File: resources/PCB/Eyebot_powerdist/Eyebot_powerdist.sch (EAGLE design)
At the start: 33 parts, among them IC3 MCP23016SO, K1 62000211622, K2 62000211622, K3 62000211622, K4 62000211622, K5 62000211622, K6 62000211622, K7 61201021621, Q1 2N2222, Q2 2N2222, Q3 2N2222

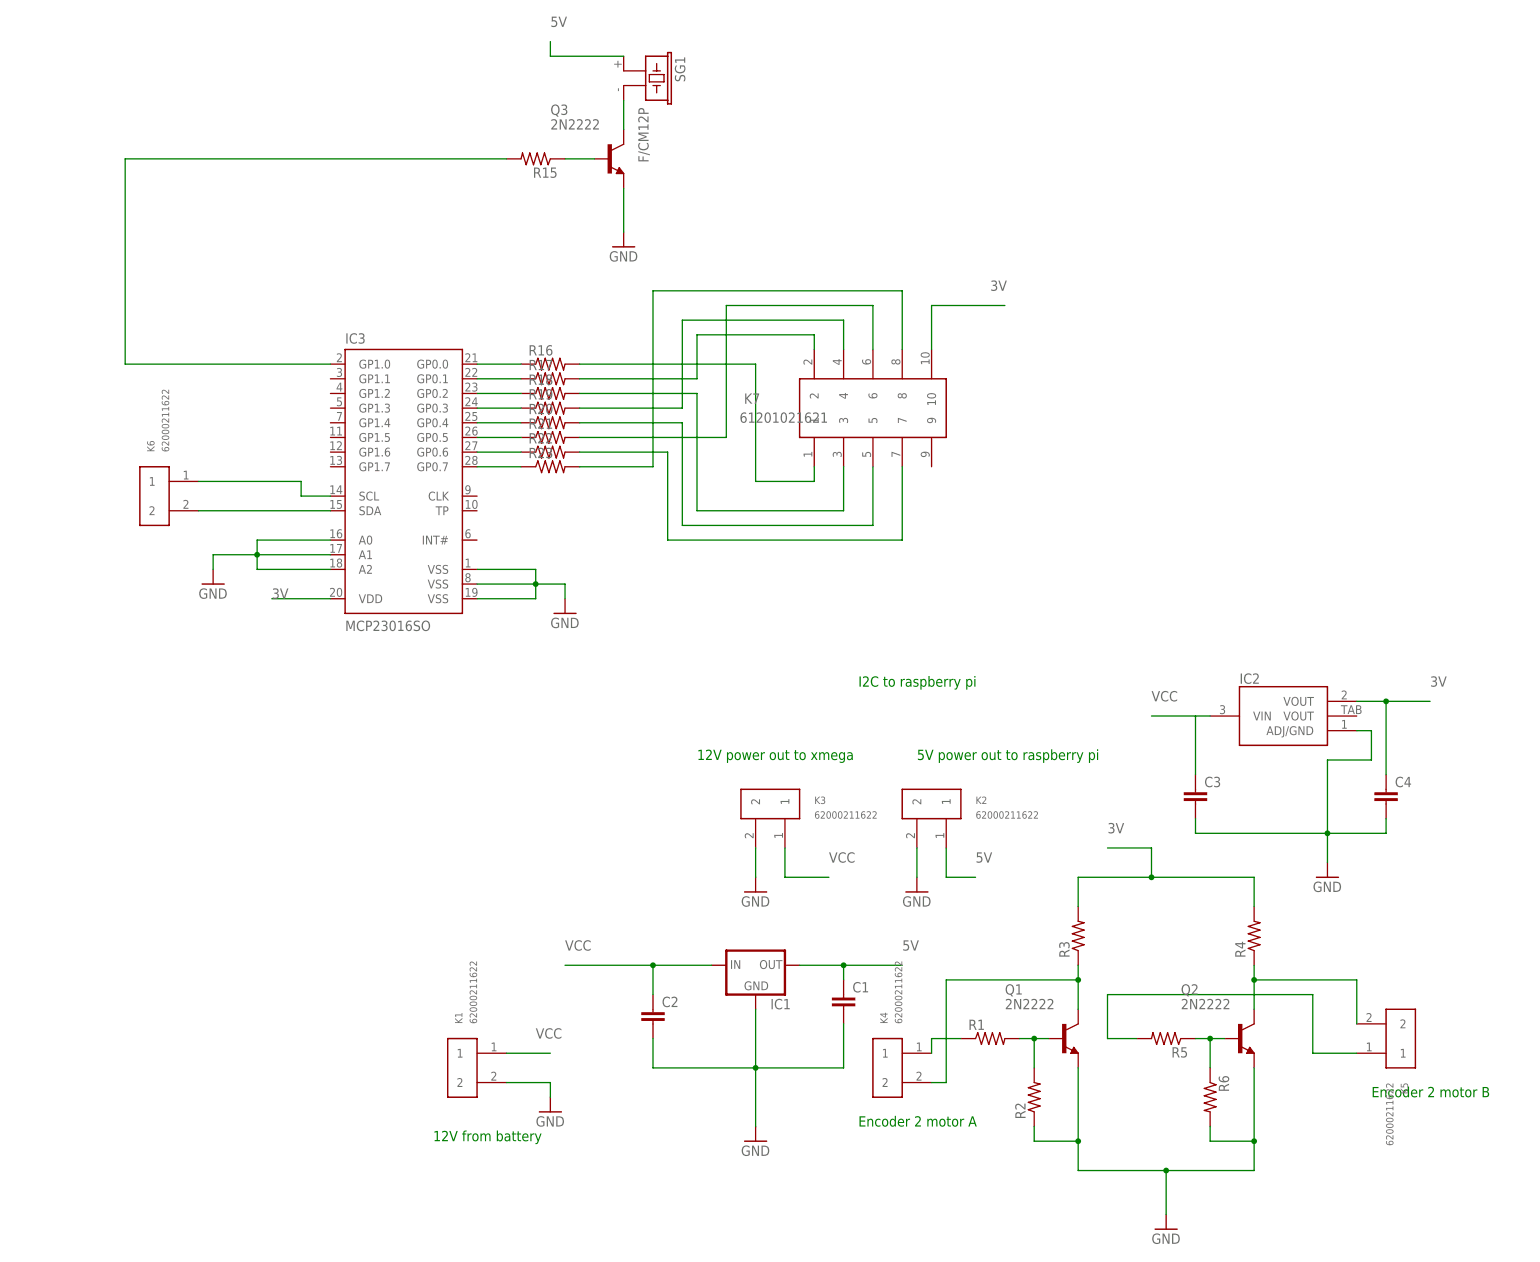
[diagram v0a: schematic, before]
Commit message: i2c chapter
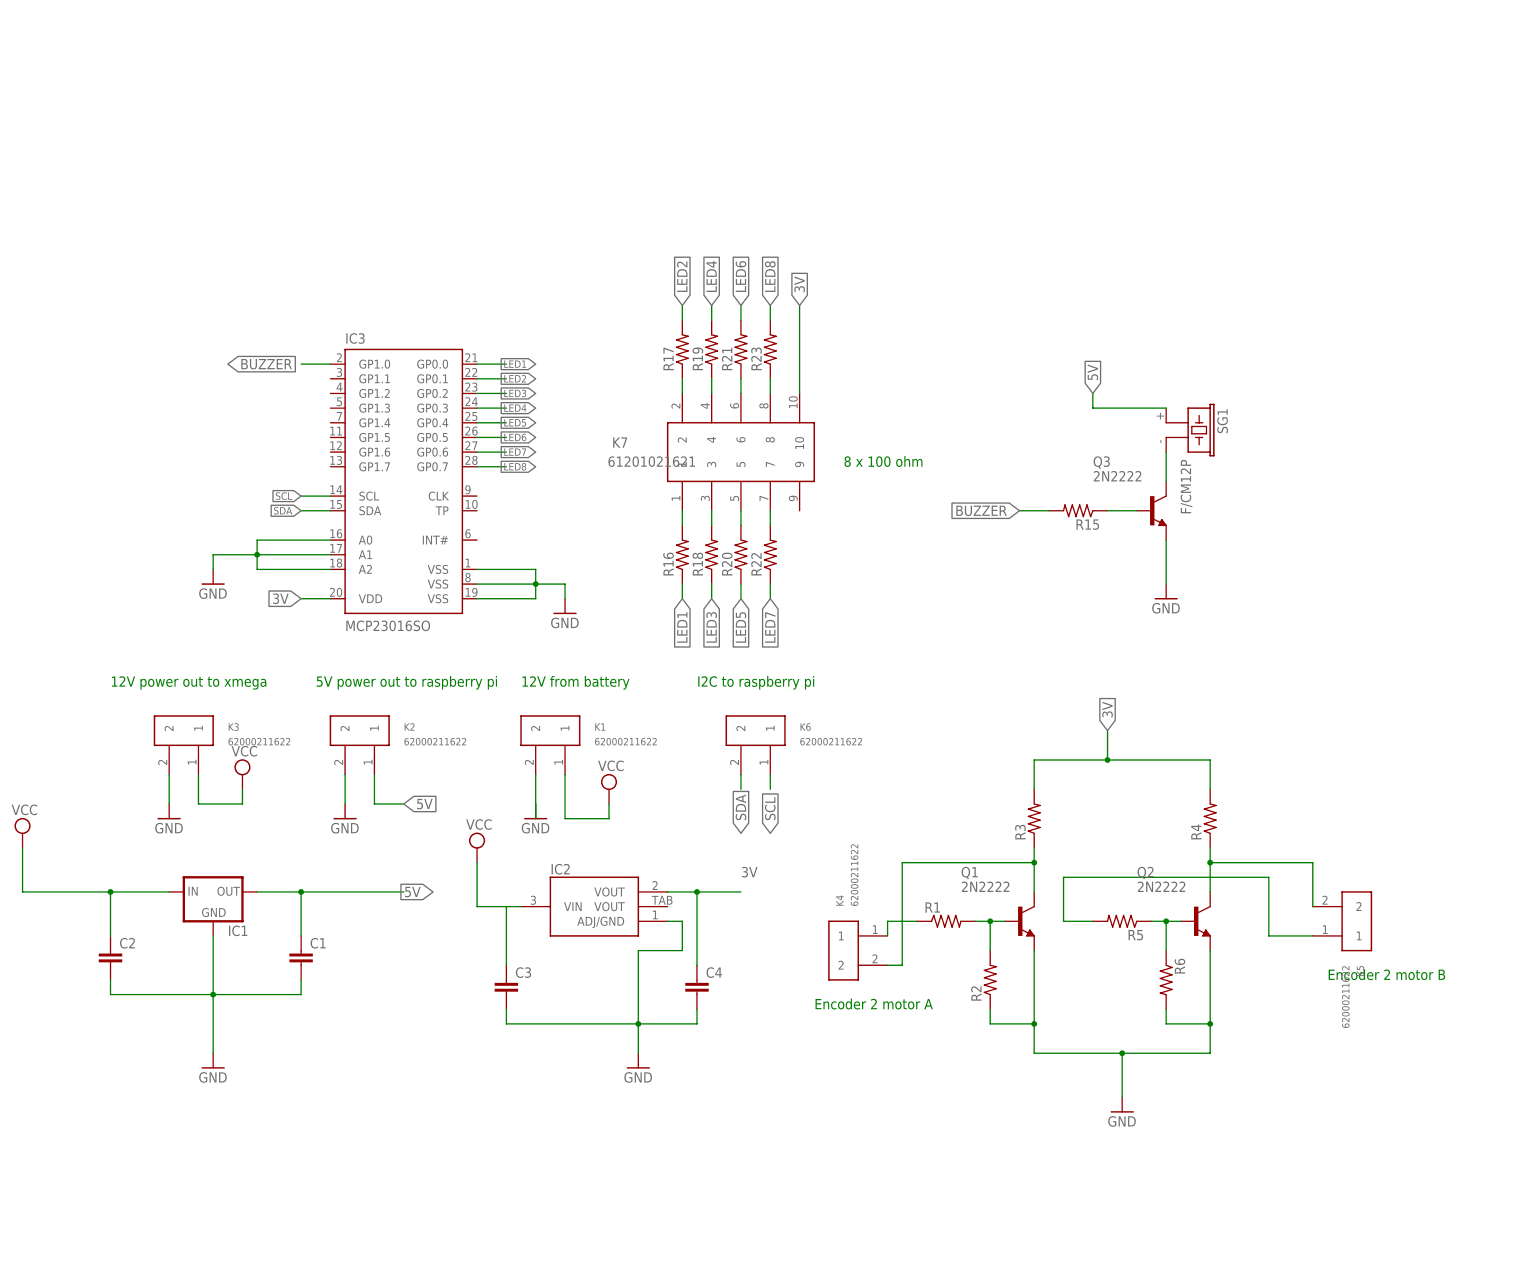
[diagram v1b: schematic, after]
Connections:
- net N$16 renamed LED5
- net N$29 renamed BUZZER
- net N$34 renamed SCL
- net N$35 renamed SDA
- net N$38 renamed LED7
- net N$42 renamed LED3
- net N$44 renamed LED1
- removed net N$12 (its old number): K7.6, R21.2
- removed net N$14 (its old number): K7.8, R23.2
- removed net N$37: IC3.GP0.7, R23.1
- removed net N$39: IC3.GP0.5, R21.1
- removed net N$41: IC3.GP0.3, R19.1
- removed net N$43: IC3.GP0.1, R17.1
- new net LED2: IC3.GP0.1, R17.2
- new net LED4: IC3.GP0.3, R19.2
- new net LED6: IC3.GP0.5, R21.2
- new net LED8: IC3.GP0.7, R23.2
- new net N$4: K7.2, R17.1
- new net N$9: K7.6, R21.1
- net N$10: now also K7.8, R23.1; no longer K7.4, R19.2
- net N$6: now also K7.4, R19.1; no longer K7.2, R17.2
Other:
- note added: "8 x 100 ohm"
- moved on the sheet: C1, C2, C3, C4, IC1, IC2, K1, K2, K3, K4, K5, K6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
